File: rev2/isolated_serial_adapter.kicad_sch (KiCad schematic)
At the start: 30 parts, among them SW3 VSEL-IN, SW4 SKAL-04H, U1 BD00IC0WHFV, U4 BD00IC0WHFV

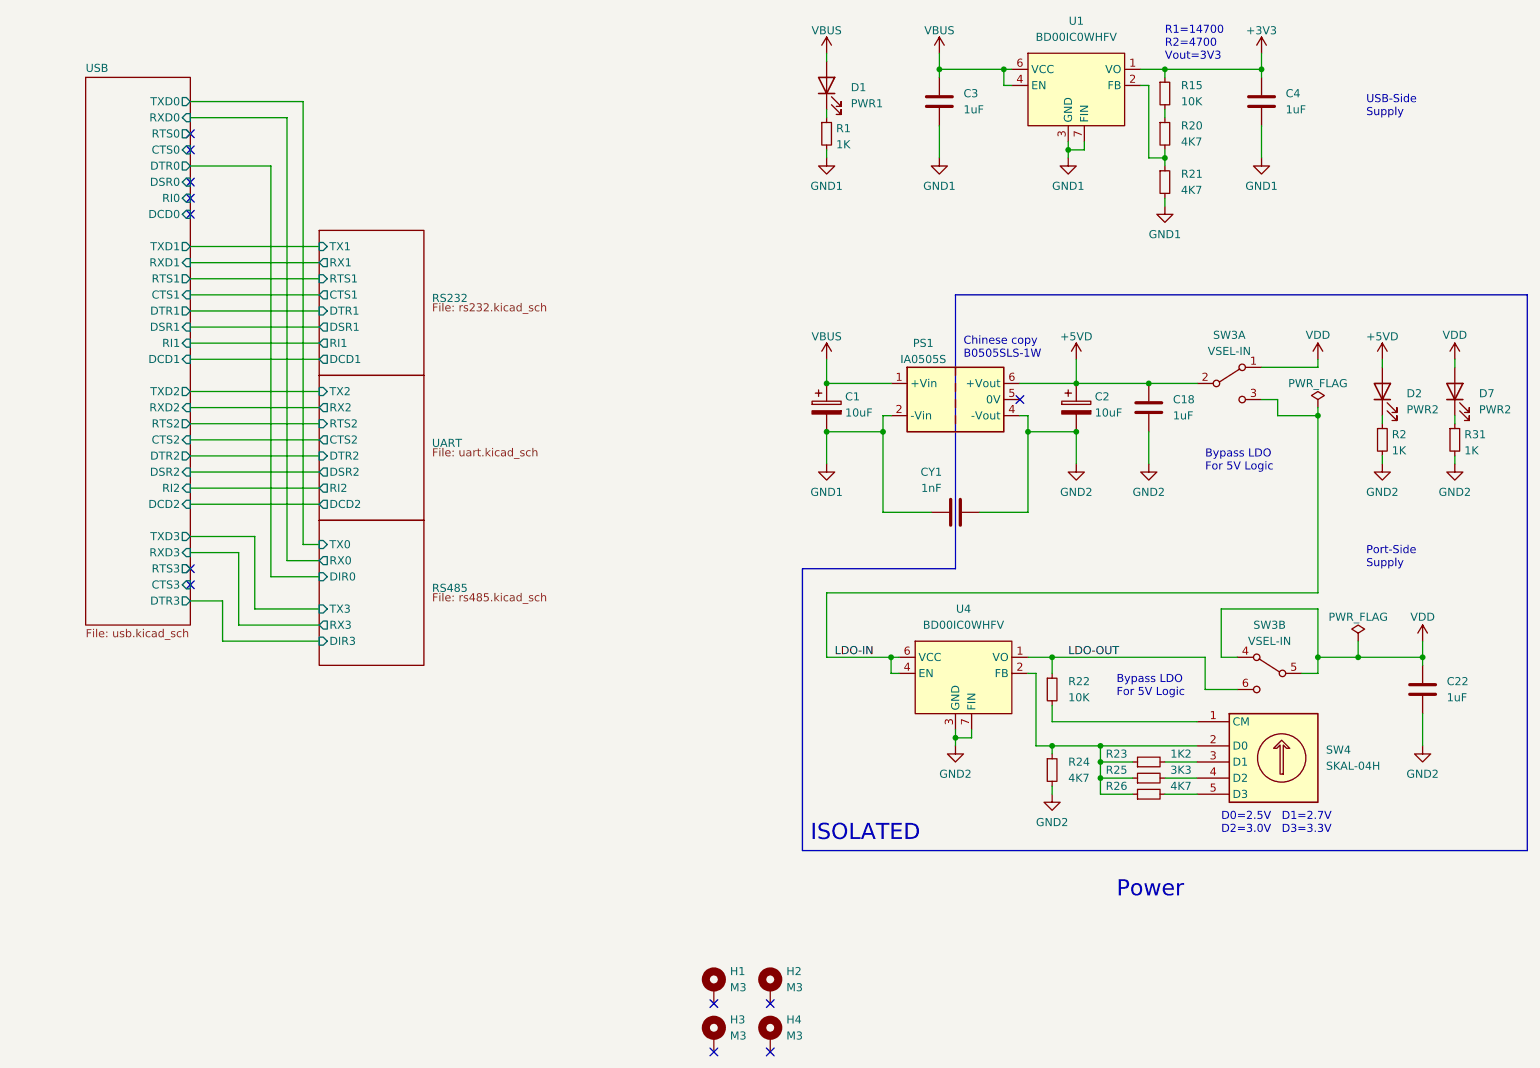
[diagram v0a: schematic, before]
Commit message: Final Rev 2 Design
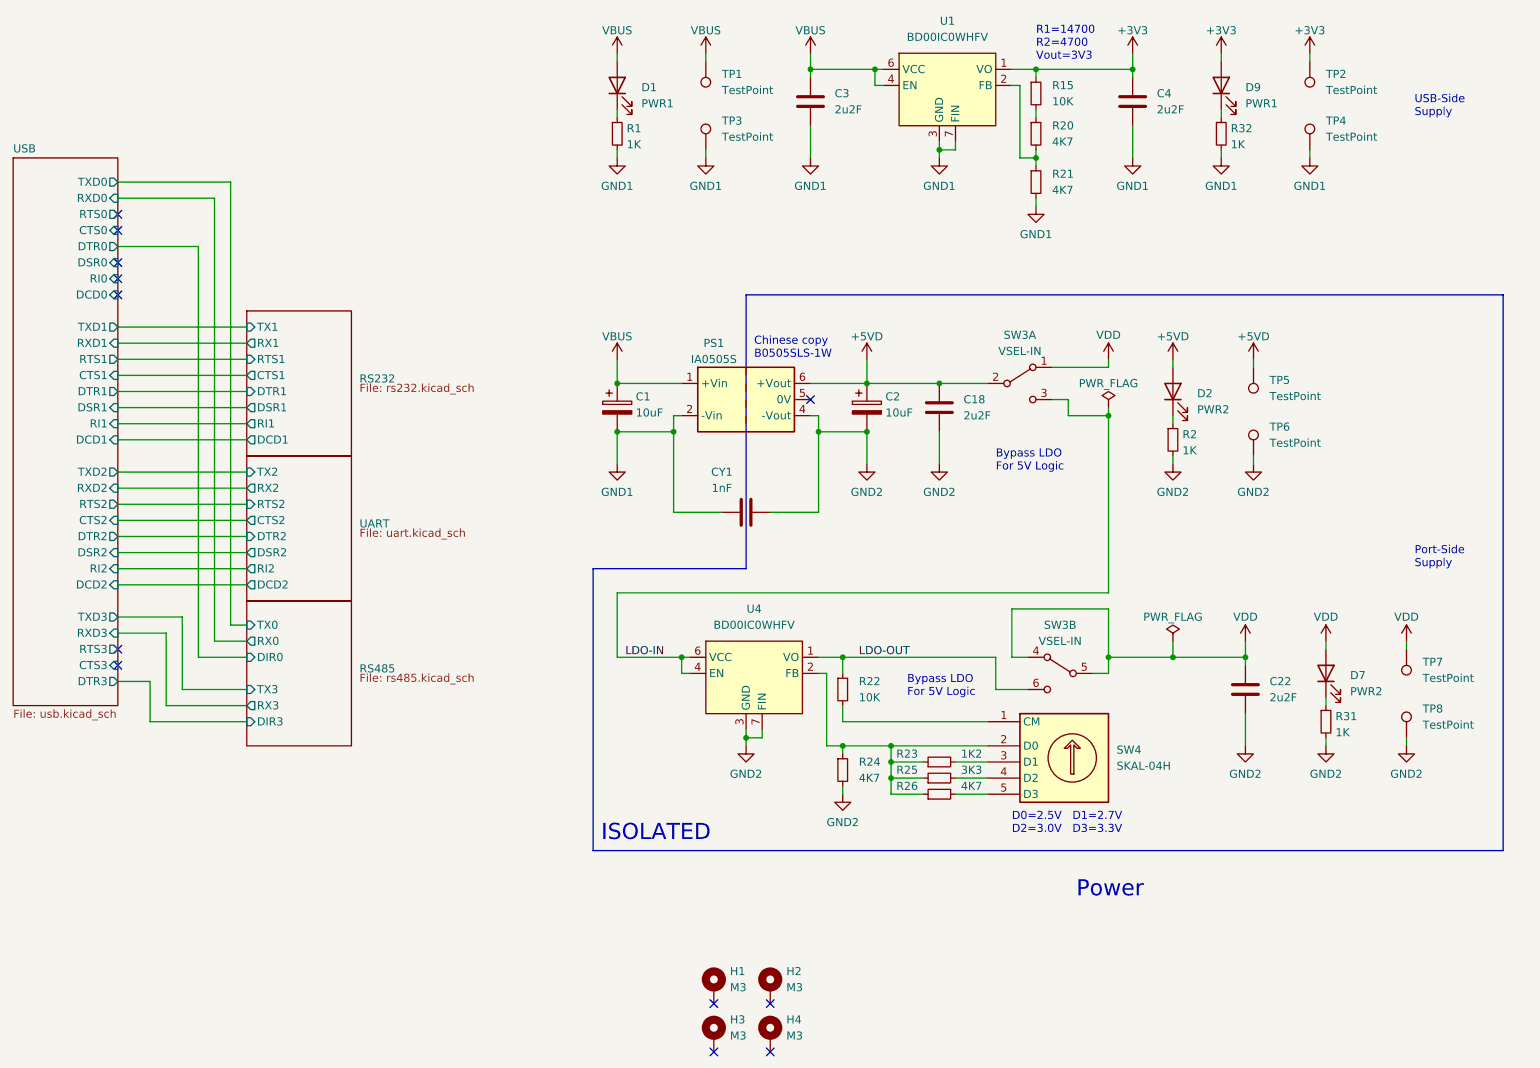
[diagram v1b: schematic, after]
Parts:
- added D9: PWR1, LED_THT:LED_D3.0mm_Clear, symbol Device:LED
- added R32: 1K, Resistor_SMD:R_0603_1608Metric, symbol Device:R_Small
- added TP1, TP2, TP3, TP4, TP5, TP6, TP7, TP8: TestPoint, TestPoint:TestPoint_Pad_D1.0mm, symbol Connector:TestPoint
- C18, C22, C3, C4: value 1uF -> 2u2F; footprint Capacitor_SMD:C_0603_1608Metric -> Capacitor_SMD:C_0805_2012Metric
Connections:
- net +3V3: now also D9.2 (A), TP2.1
- net +5VD: now also TP5.1
- net GND1: now also R32.2, TP3.1, TP4.1
- net GND2: now also TP6.1, TP8.1
- net VBUS: now also TP1.1
- net VDD: now also TP7.1
- new net: D9.1 (K), R32.1
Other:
- moved on the sheet: C1, C18, C2, C22, C3, C4, CY1, D1, D2, D7, PS1, R1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
